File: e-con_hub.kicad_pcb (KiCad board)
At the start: 2 copper layers, 55 x 25 mm, 7 parts, among them J7 XG4A-1031

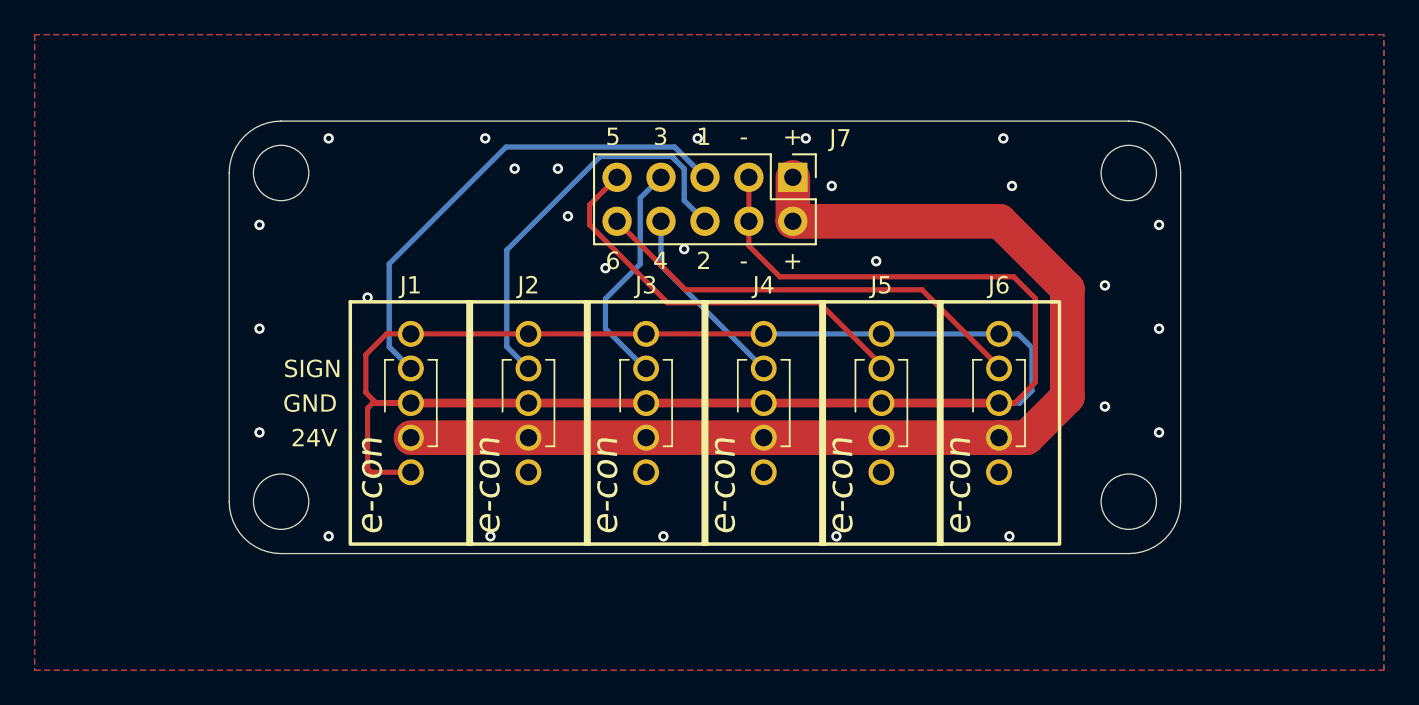
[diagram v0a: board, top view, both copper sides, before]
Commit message: パターンを微修正
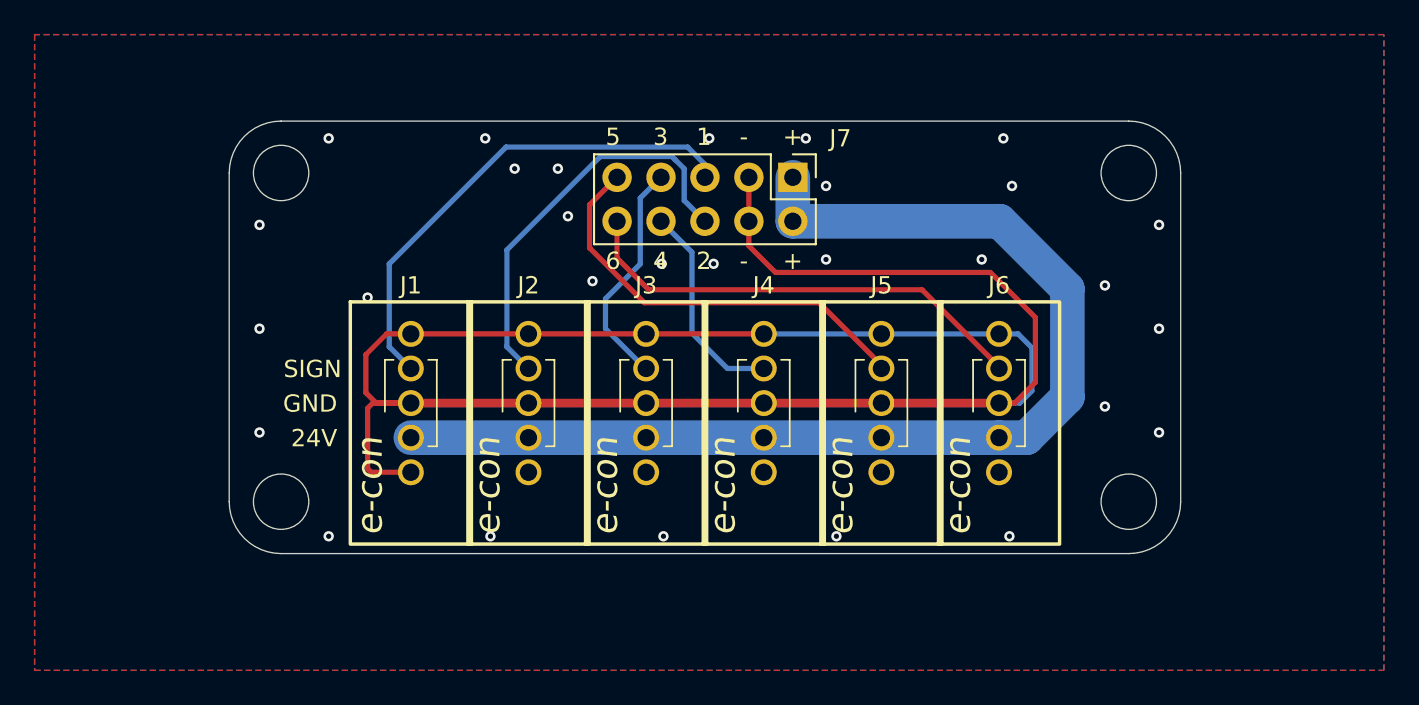
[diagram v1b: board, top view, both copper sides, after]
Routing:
- net Net-(J7-Pin_10): track 25.6 -> 26.8 mm
- net Net-(J7-Pin_8): track 11.0 -> 12.2 mm
- net Net-(J7-Pin_9): track 23.8 -> 24.6 mm
- net GND: track 121.0 -> 120.4 mm, vias 27 -> 29
